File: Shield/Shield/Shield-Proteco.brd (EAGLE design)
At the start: 114.7 x 79.4 mm, 54 parts, among them Q2 TIP41C

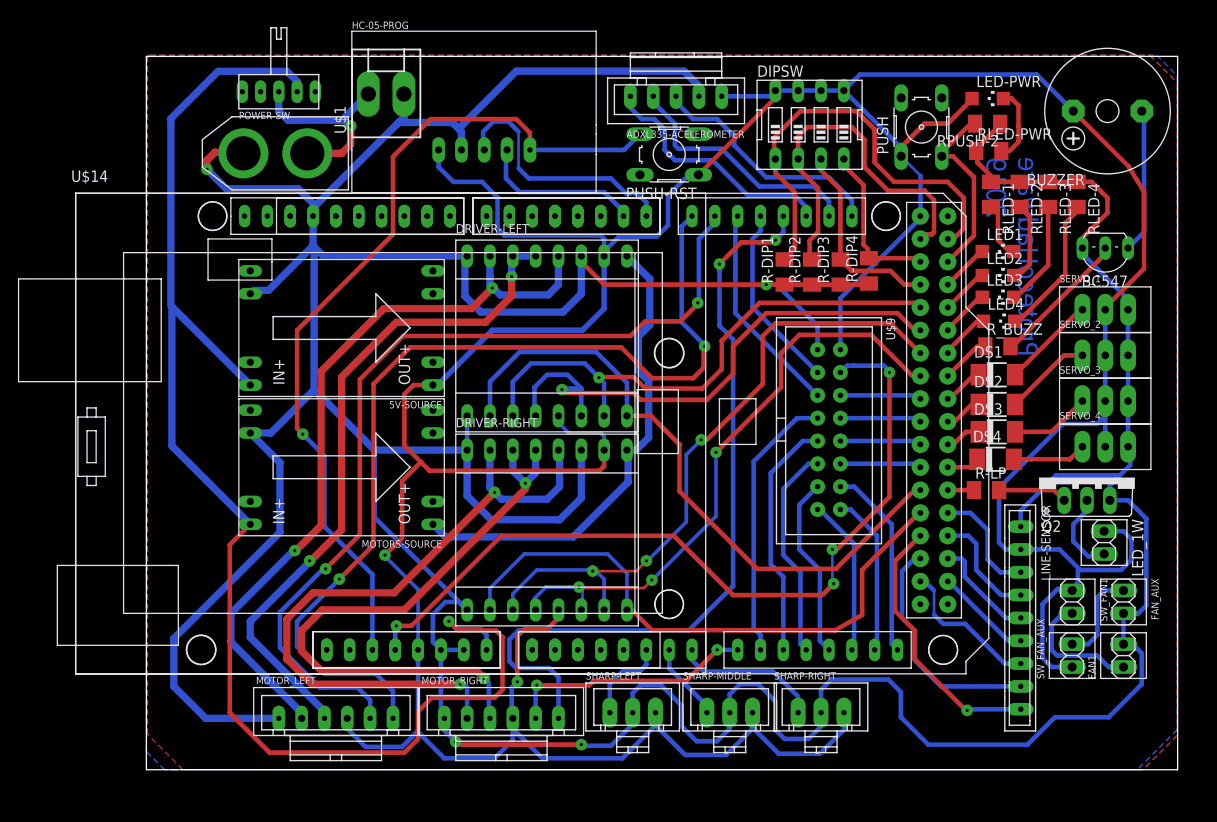
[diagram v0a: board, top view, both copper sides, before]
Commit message: Shield Terminada
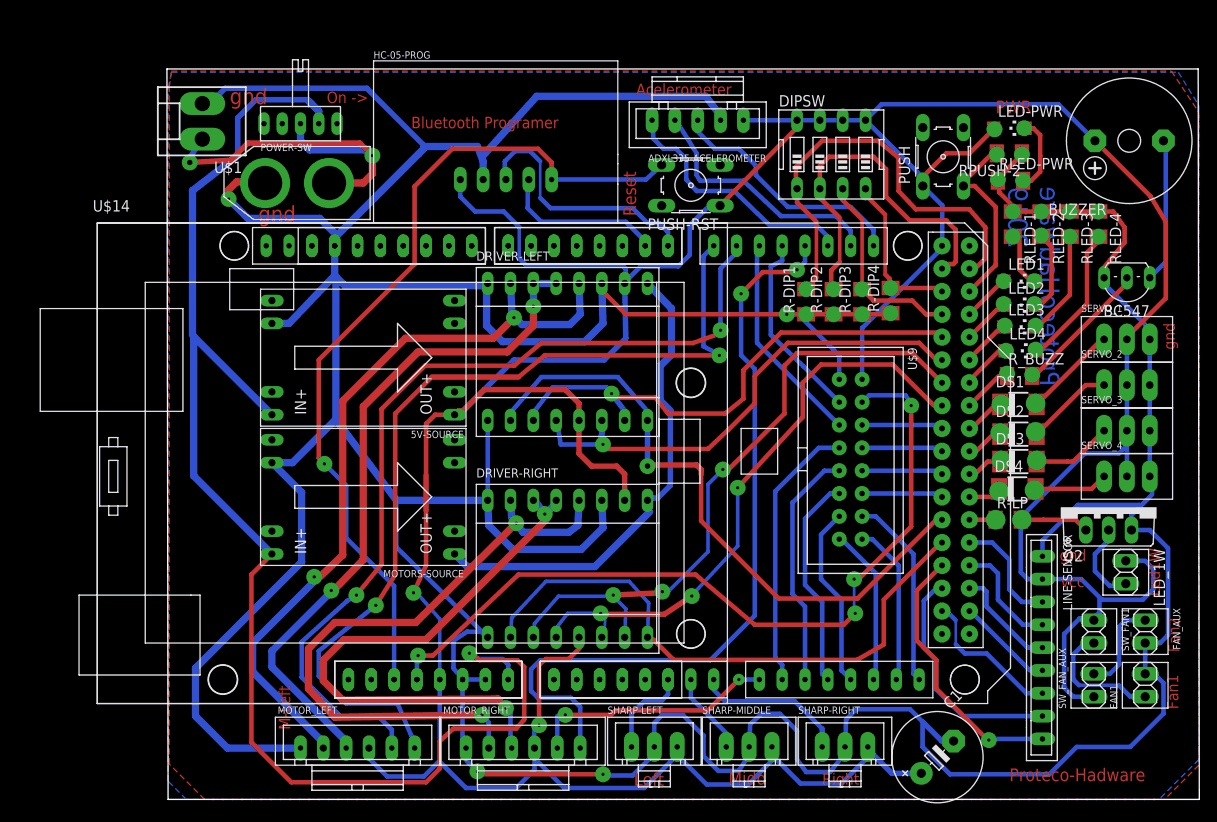
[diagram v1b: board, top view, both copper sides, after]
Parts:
- added C1: (no value), rcl:E5-10,5
- moved U$1 20.7 mm to (2.41, 73.3), turned to 90 degrees
- moved DRIVER-RIGHT 6.04 mm to (43.1, 22.2)
- moved SHARP-RIGHT 4.65 mm to (73.9, 3.68)
- moved SHARP-LEFT 4.51 mm to (52.7, 3.68)
- moved SHARP-MIDDLE 4.38 mm to (63.2, 3.68)
- moved POWER-SW 4.30 mm to (13.3, 73.0)
- moved PUSH-RST 4.19 mm to (56.8, 66.2)
- moved LED_1W 4.09 mm to (105.2, 23.1)
- moved LINE-SENSOR 4.09 mm to (95.9, 14.7)
- moved Q2 4.09 mm to (103.3, 30.4)
- moved R-DIP2 4.09 mm to (72.6, 53.2)
- moved RLED-3 4.09 mm to (98.9, 61.8)
- moved RLED-4 4.09 mm to (102.1, 61.8)
- moved U$9 4.09 mm to (74.5, 35.7)
- moved HC-05-PROG 4.09 mm to (34.9, 70.9)
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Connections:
- net GND: now also C1.-
- net VCC: now also C1.+
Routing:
- net GND: track 553.1 -> 584.7 mm
- net N$134: track 22.3 -> 42.6 mm, vias 1 -> 2
- net ENC1-LEFT: track 107.3 -> 100.8 mm
- net OUT2-MOTOR-RIGHT: track 69.0 -> 64.9 mm
- net IN2-MOTOR-LEFT: track 61.7 -> 58.3 mm
- net IN1-MOTOR-LEFT: track 62.0 -> 58.8 mm
- net OUT1-MOTOR-RIGHT: track 75.5 -> 72.5 mm
- net VCC: track 449.9 -> 452.9 mm
- net 3V3: track 91.8 -> 90.3 mm
- net OUT1-MOTOR-LEFT: track 84.1 -> 85.0 mm
- net IN1-MOTOR-RIGHT: track 74.5 -> 73.7 mm
- net INT: track 27.8 -> 28.5 mm
- net 6V-DC-3A: track 53.7 -> 54.3 mm
- net SHARP-RIGHT: track 16.4 -> 17.0 mm
- net RX2: track 20.8 -> 21.4 mm
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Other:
- board size 114.7 x 79.4 mm -> 114.9 x 81.3 mm
- board text added: "Acelerometer"
- board text added: "Bluetooth Programer"
- board text added: "Fan1"
- board text added: "Fan2"
- board text added: "Led1W"
- board text added: "Left"
- board text added: "M-Left"
- board text added: "Midd"
- board text added: "On ->"
- board text added: "PWR"
- board text added: "Proteco-Hadware"
- board text added: "Reset"
- board text added: "Right"
- board text added: "gnd"
- board text added: "vcc"
